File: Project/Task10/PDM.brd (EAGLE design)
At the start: 101.3 x 78.7 mm, 43 parts

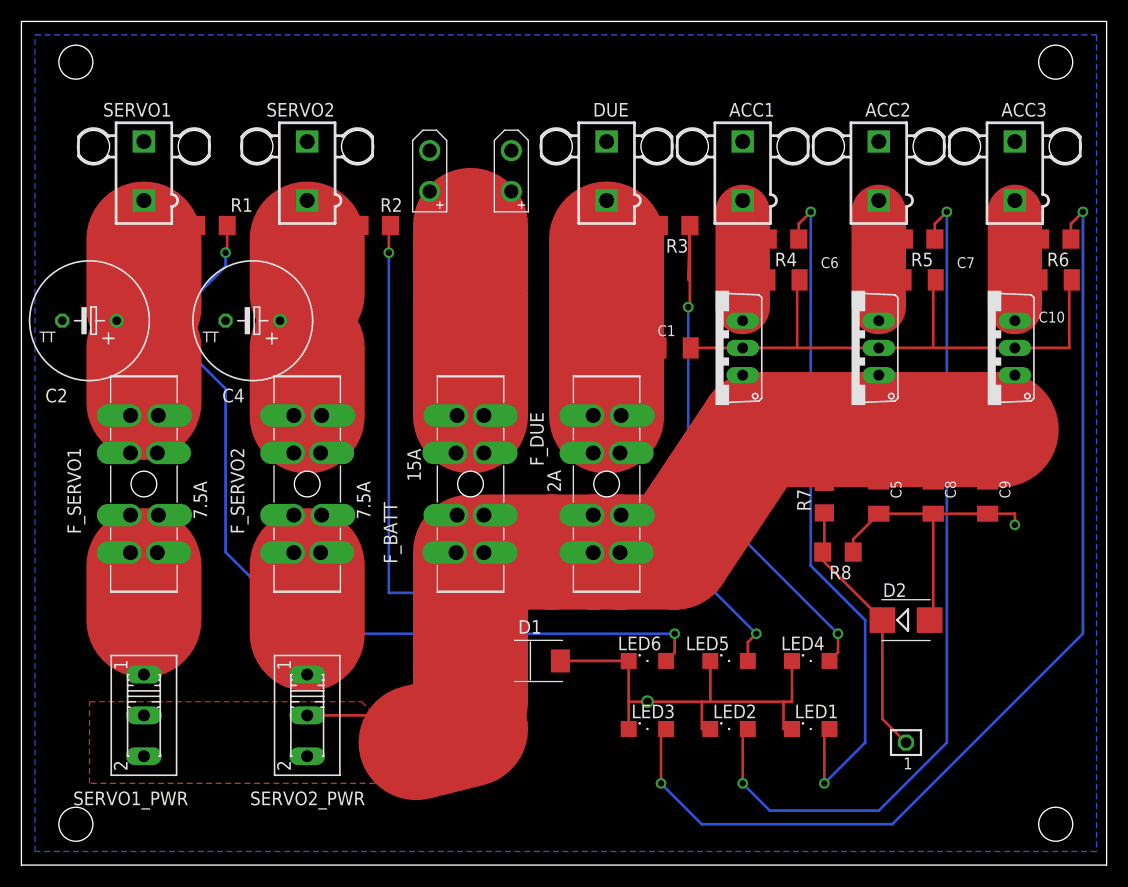
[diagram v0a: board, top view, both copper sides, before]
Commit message: More PDM work
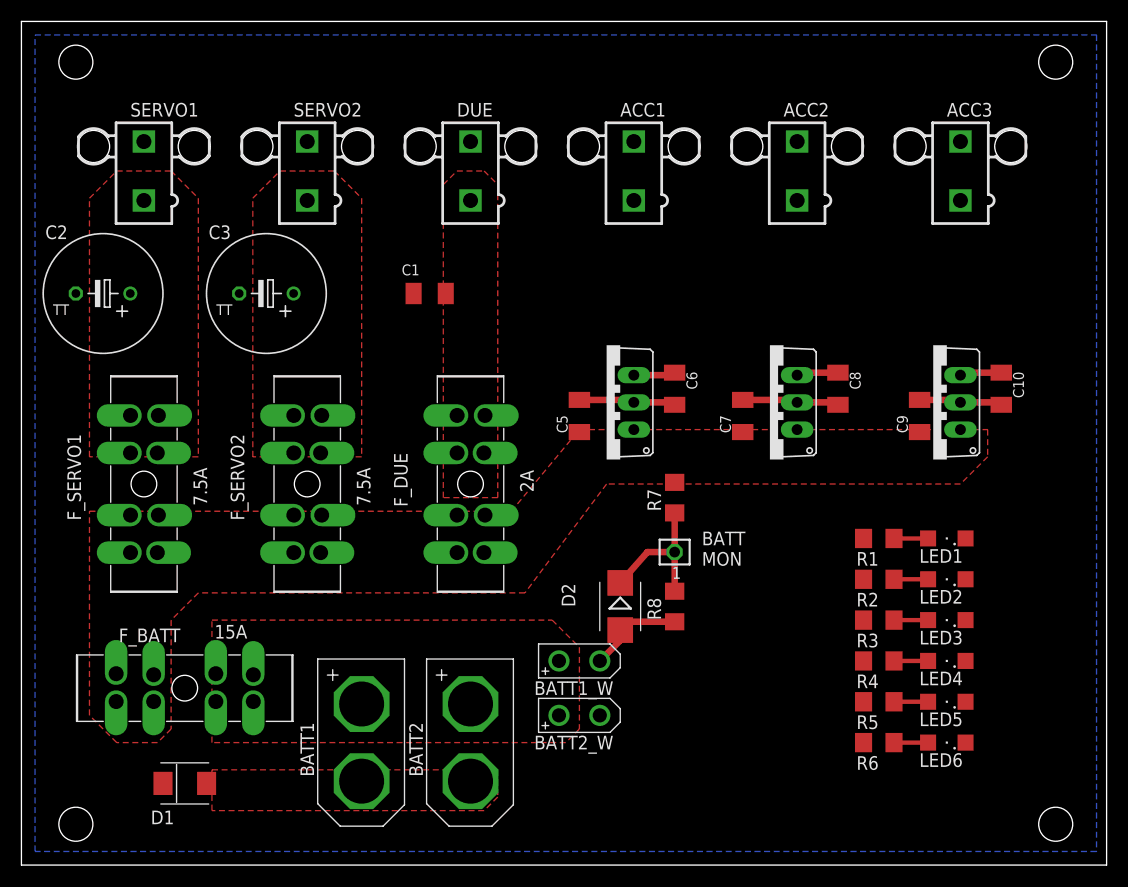
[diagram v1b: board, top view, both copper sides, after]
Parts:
- removed C4: (no value), rcl:TT5D11
- removed SERVO1_PWR, SERVO2_PWR: (no value), switch:255SB
- removed U$4, U$5: CON_XT60-PIGTAIL, MRSDTeamB:CON_XT60_PIGTAIL
- added BATT1, BATT2: (no value), MRSDTeamB:CON_XT60_PCB_MOUNT
- added BATT1_W, BATT2_W: (no value), MRSDTeamB:CON_XT60_PIGTAIL
- added C3: (no value), rcl:TT5D11
- moved R1 68.7 mm to (80.0, 30.5)
- moved R2 57.4 mm to (80.0, 26.7)
- moved R6 49.8 mm to (80.0, 11.4)
- moved R5 43.3 mm to (80.0, 15.2)
- moved R3 41.5 mm to (80.0, 22.9)
- moved R4 40.4 mm to (80.0, 19.1)
- moved D1 34.9 mm to (15.2, 7.62)
- moved F_BATT 32.8 mm to (15.2, 16.5), turned to 180 degrees
- moved LED3 29.7 mm to (86.4, 22.9), turned to 180 degrees
- moved C5 29.0 mm to (52.1, 41.9), turned to 90 degrees
- moved LED6 29.0 mm to (86.4, 11.4), turned to 180 degrees
- moved BAT_MON 28.0 mm to (61.0, 29.2)
- moved D2 26.7 mm to (55.9, 24.1), turned to 270 degrees
- moved LED2 24.7 mm to (86.4, 26.7), turned to 180 degrees
- moved C1 23.4 mm to (38.1, 53.3), turned to 180 degrees
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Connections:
- removed net N$12: F_SERVO1.A1, F_SERVO1.A2, F_SERVO1.A3, F_SERVO1.A4, SERVO1_PWR.1
- removed net N$14: F_SERVO2.A1, F_SERVO2.A2, F_SERVO2.A3, F_SERVO2.A4, SERVO2_PWR.1
- net GND: now also BATT1.V-, BATT1_W.V-, BATT2.V-, BATT2_W.V-, C3.-; no longer C4.-, U$4.V-, U$5.V-
- net N$1: now also C3.+; no longer C4.+
- net N$11: now also LED3.A; no longer LED4.A
- net N$13: now also LED4.A; no longer LED1.A
- net N$16: now also LED5.A; no longer LED2.A
- net N$2: now also BATT1.V+, BATT1_W.V+, BATT2.V+, BATT2_W.V+; no longer U$4.V+, U$5.V+
- net N$22: now also LED6.A; no longer LED3.A
- net N$5: now also LED1.A; no longer LED6.A
- net N$8: now also LED2.A; no longer LED5.A
- net N$9: now also C8.1; no longer C7.1
- net V_SUPPLY: now also C7.1, F_SERVO1.A1, F_SERVO1.A2, F_SERVO1.A3, F_SERVO1.A4, F_SERVO2.A1, F_SERVO2.A2, F_SERVO2.A3, F_SERVO2.A4; no longer C8.1, SERVO1_PWR.2, SERVO2_PWR.2
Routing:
- net V_SUPPLY: track 151.4 -> 0.00 mm
- net N$22: track 96.2 -> 3.18 mm, vias 2 -> 0
- net GND: track 126.4 -> 36.3 mm, vias 2 -> 0
- net N$5: track 81.6 -> 3.18 mm, vias 2 -> 0
- net N$16: track 80.8 -> 3.18 mm, vias 2 -> 0
- net N$29: track 73.4 -> 0.00 mm
- net N$8: track 73.2 -> 3.18 mm, vias 2 -> 0
- net N$13: track 65.6 -> 3.18 mm, vias 2 -> 0
- net N$4: track 50.3 -> 0.00 mm
- net N$11: track 51.9 -> 3.18 mm, vias 2 -> 0
- net N$15: track 47.9 -> 0.00 mm
- net N$1: track 46.8 -> 0.00 mm
- net N$2: track 37.7 -> 0.00 mm
- net N$14: track 21.3 -> 0.00 mm
- net N$12: track 21.2 -> 0.00 mm
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- added copper zone on layer 1, net GND
- added copper zone on layer 1, net N$1
- added copper zone on layer 1, net N$15
- added copper zone on layer 1, net N$2
- added copper zone on layer 1, net N$4
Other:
- board text added: "BATT MON"
- board text removed: "Acc1"
- board text removed: "Acc2"
- board text removed: "Acc3"
- board text removed: "Battery"
- board text removed: "Battery Monitoring"
- board text removed: "DUE"
- board text removed: "SRV1"
- board text removed: "SRV2"
